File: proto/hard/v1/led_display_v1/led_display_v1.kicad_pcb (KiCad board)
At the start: 2 copper layers, 87 x 50 mm, 100 parts, among them U1 LCD_2.8_SPI, U2 74HCT595, U3 74HCT595, U4 74HCT595

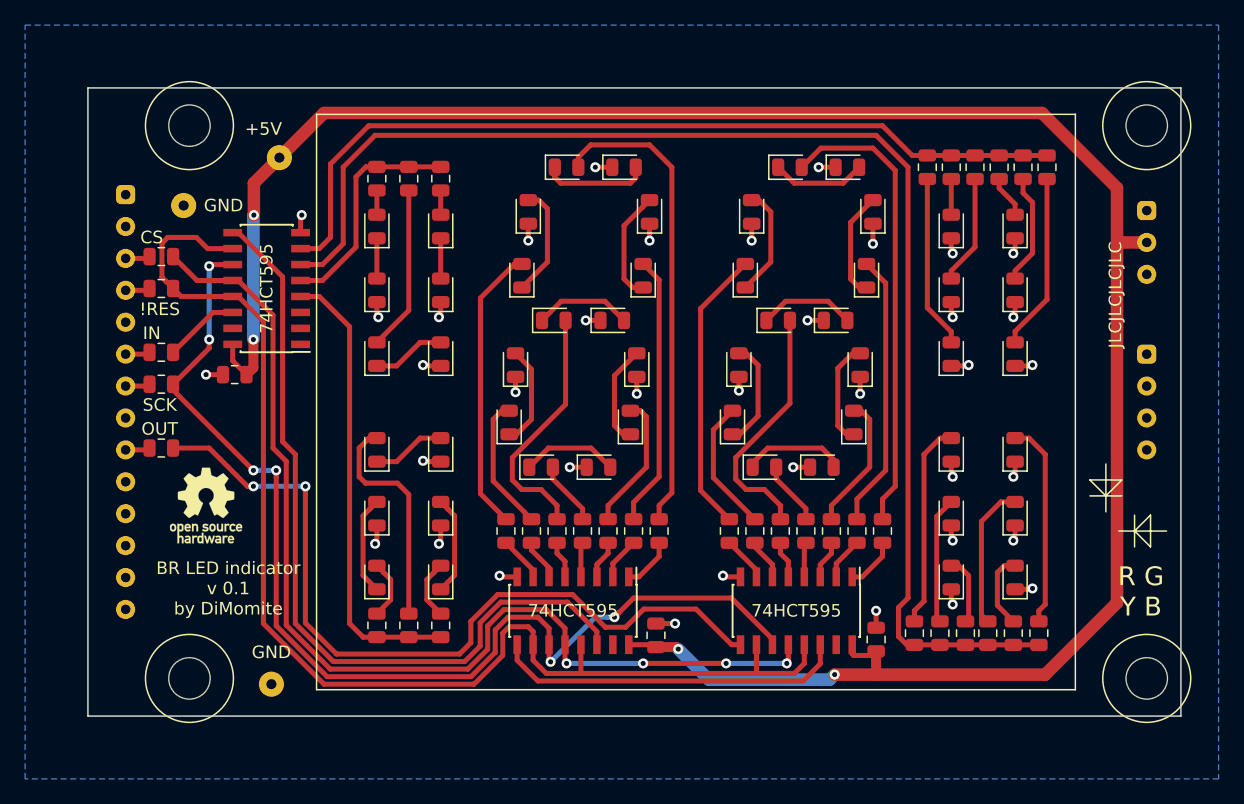
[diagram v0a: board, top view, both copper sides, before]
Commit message: Generated gerbers for LED indicator.
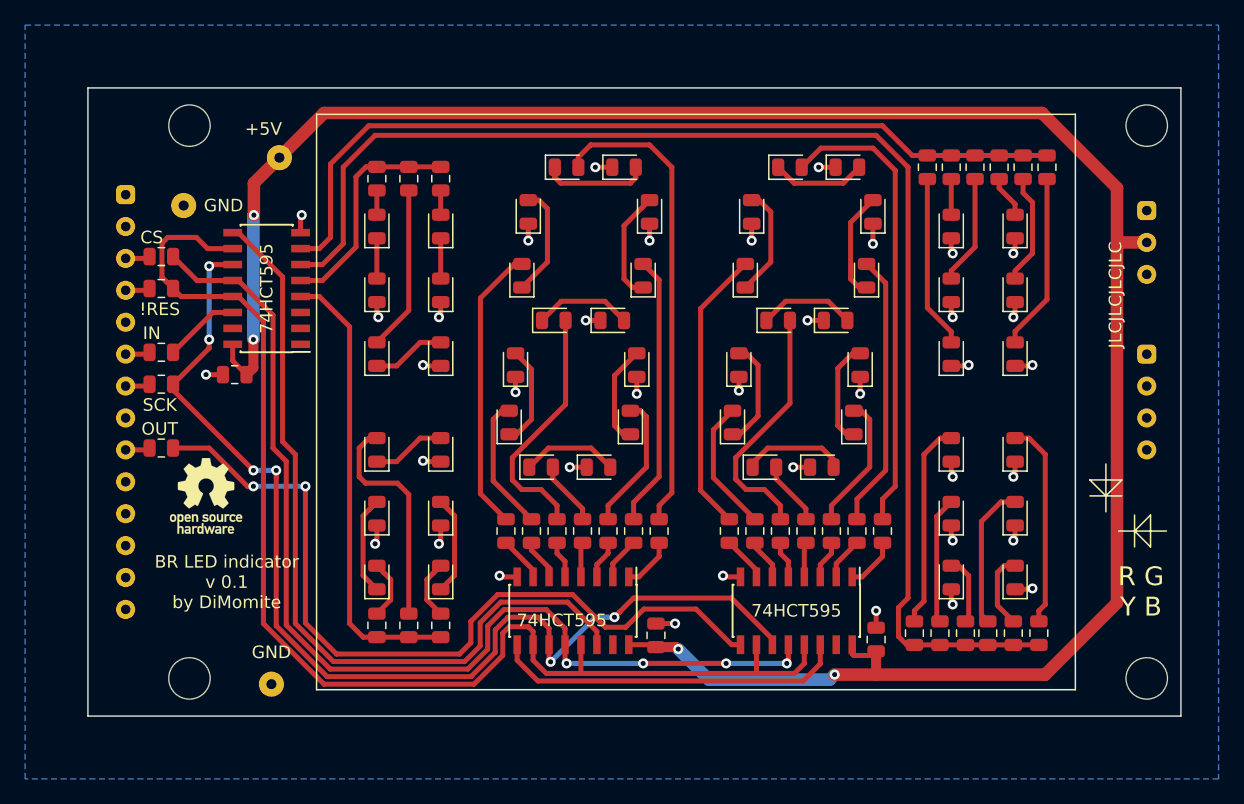
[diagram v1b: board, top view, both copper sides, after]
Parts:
- moved REF** 0.76 mm to (109.4, 82.5)
